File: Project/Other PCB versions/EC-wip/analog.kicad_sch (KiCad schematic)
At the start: 22 parts, among them U4 74HC4051, U5 OPA350, U6 74HC4051

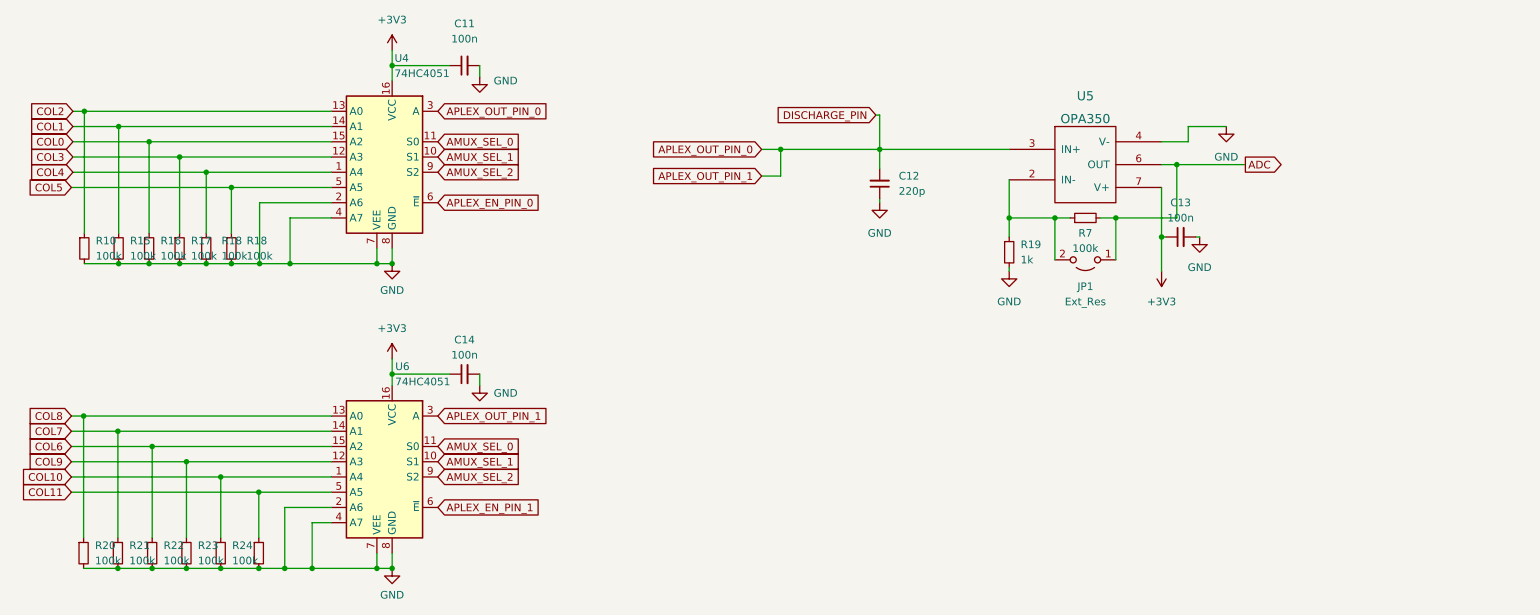
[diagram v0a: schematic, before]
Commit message: EC progress
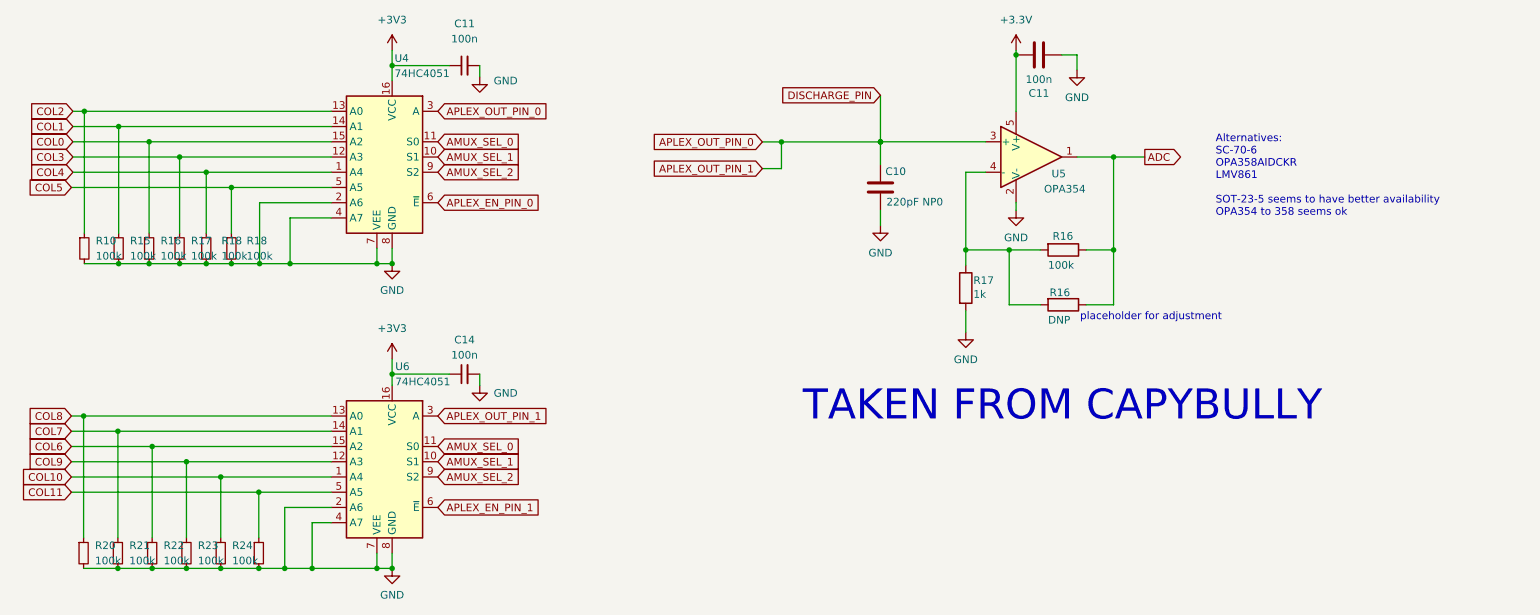
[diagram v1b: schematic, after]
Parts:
- removed C12: 220p, Capacitor_SMD:C_0402_1005Metric, symbol Device:C_Small
- removed C13: 100n, Capacitor_SMD:C_0402_1005Metric, symbol Device:C_Small
- removed JP1: Ext_Res, Resistor_SMD:R_0603_1608Metric_Pad0.98x0.95mm_HandSolder, symbol Jumper:Jumper_2_Open
- removed R19: 1k, Resistor_SMD:R_0402_1005Metric, symbol Device:R_Small
- removed R7: 100k, Resistor_SMD:R_0402_1005Metric, symbol Device:R_Small
- removed U5: OPA350, Package_SO:SOIC-8_3.9x4.9mm_P1.27mm, symbol cipulot_parts:OPA350
- added C10: 220pF NP0, Capacitor_SMD:C_0402_1005Metric, symbol Device:C
- added C11: 100n, Capacitor_SMD:C_0402_1005Metric, symbol Device:C
- added R16: 100k, Resistor_SMD:R_0402_1005Metric, symbol Device:R
- added R16: DNP, Resistor_SMD:R_0402_1005Metric, symbol Device:R
- added R17: 1k, Resistor_SMD:R_0402_1005Metric, symbol Device:R
- added U5: OPA354, Package_TO_SOT_SMD:SOT-23-5, symbol Amplifier_Operational:OPA340NA
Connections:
- net +3V3: now also C11.2, U5.5 (V+)
- net ADC: now also R16.1, R16.1, U5.1
- net APLEX_OUT_PIN_0: now also C10.1, U5.3 (+)
- net GND: now also C10.2, C11.1, R17.2, U5.2 (V-)
- new net: R16.2, R16.2, R17.1, U5.4 (-)
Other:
- note added: "Alternatives: SC-70-6 OPA358AIDCKR LMV861 SOT-23-5 seems to have better availability OPA354 to 358 seems ok"
- note added: "TAKEN FROM CAPYBULLY"
- note added: "placeholder for adjustment"

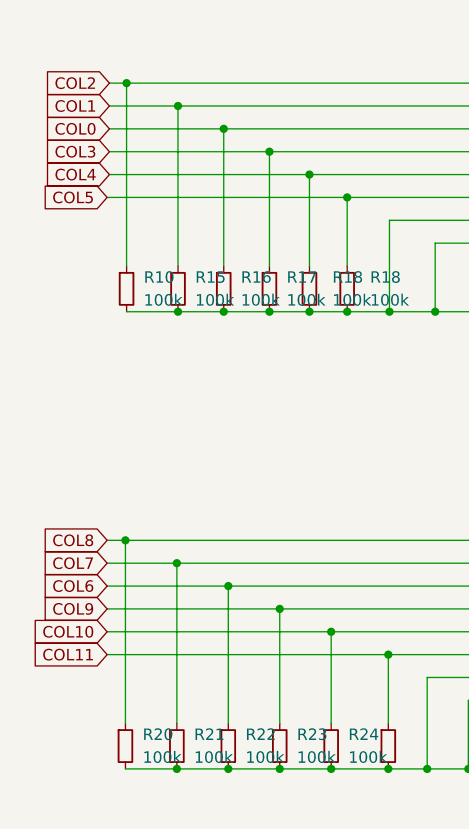
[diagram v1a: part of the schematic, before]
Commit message: two different pcb versions
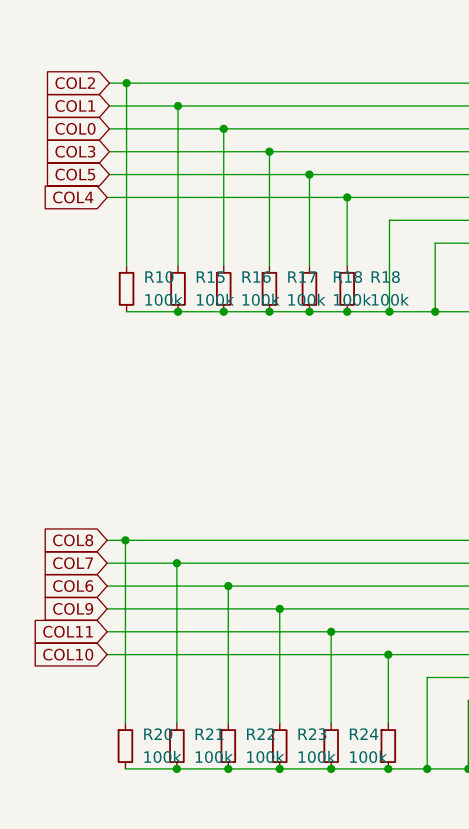
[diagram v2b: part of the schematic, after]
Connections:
- net COL10: now also R25.1, U6.5 (A5); no longer R24.1, U6.1 (A4)
- net COL11: now also R24.1, U6.1 (A4); no longer R25.1, U6.5 (A5)
- net COL4: now also R18.1, U4.5 (A5); no longer R18.1, U4.1 (A4)
- net COL5: now also R18.1, U4.1 (A4); no longer R18.1, U4.5 (A5)
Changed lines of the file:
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@@
     )
   )
-  (global_label "COL10" (shape input) (at 55.88 101.6 180) (fields_autoplaced)
+  (global_label "COL10" (shape input) (at 55.88 104.14 180) (fields_autoplaced)
     (effects (font (size 1.27 1.27)) (justify right))
-    (property "Intersheetrefs" "${INTERSHEET_REFS}" (at 46.9266 101.6 0)
+    (property "Intersheetrefs" "${INTERSHEET_REFS}" (at 46.9266 104.14 0)
       (effects (font (size 1.27 1.27)) (justify right) hide)
     )
@@
     )
   )
-  (global_label "COL4" (shape input) (at 56.134 50.8 180) (fields_autoplaced)
+  (global_label "COL4" (shape input) (at 55.88 53.34 180) (fields_autoplaced)
     (effects (font (size 1.27 1.27)) (justify right))
-    (property "Intersheetrefs" "${INTERSHEET_REFS}" (at 48.8828 50.8794 0)
+    (property "Intersheetrefs" "${INTERSHEET_REFS}" (at 48.6288 53.4194 0)
       (effects (font (size 1.27 1.27)) (justify right) hide)
     )
@@
     )
   )
-  (global_label "COL11" (shape input) (at 55.88 104.14 180) (fields_autoplaced)
+  (global_label "COL11" (shape input) (at 55.88 101.6 180) (fields_autoplaced)
     (effects (font (size 1.27 1.27)) (justify right))
-    (property "Intersheetrefs" "${INTERSHEET_REFS}" (at 46.9266 104.14 0)
+    (property "Intersheetrefs" "${INTERSHEET_REFS}" (at 46.9266 101.6 0)
       (effects (font (size 1.27 1.27)) (justify right) hide)
     )
   )
-  (global_label "COL5" (shape input) (at 55.88 53.34 180) (fields_autoplaced)
+  (global_label "COL5" (shape input) (at 56.134 50.8 180) (fields_autoplaced)
     (effects (font (size 1.27 1.27)) (justify right))
-    (property "Intersheetrefs" "${INTERSHEET_REFS}" (at 48.6288 53.4194 0)
+    (property "Intersheetrefs" "${INTERSHEET_REFS}" (at 48.8828 50.8794 0)
       (effects (font (size 1.27 1.27)) (justify right) hide)
     )
